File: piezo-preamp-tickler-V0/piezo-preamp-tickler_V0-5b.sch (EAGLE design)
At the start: 22 parts, among them IC1 TLC272, Q4 2N5484

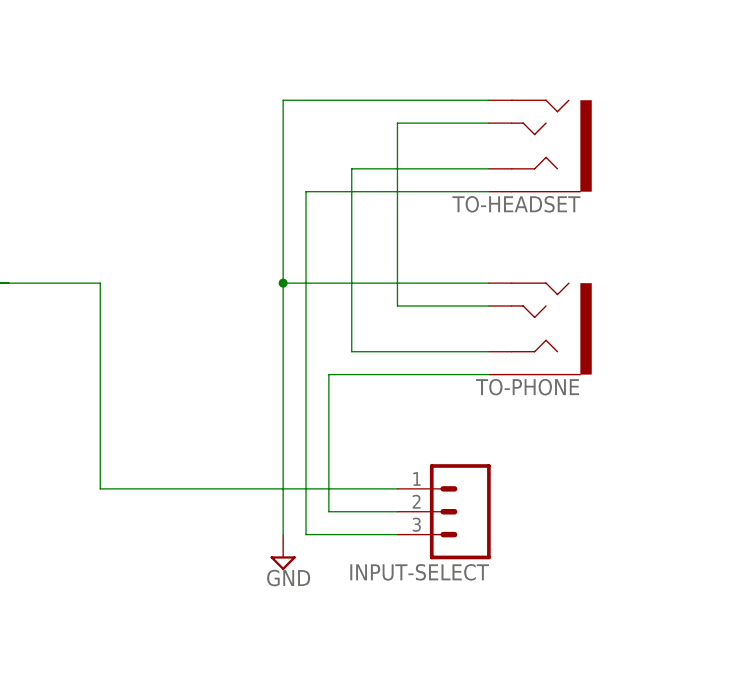
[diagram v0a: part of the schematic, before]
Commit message: changes to piezo-preamp-tickler-V0-5
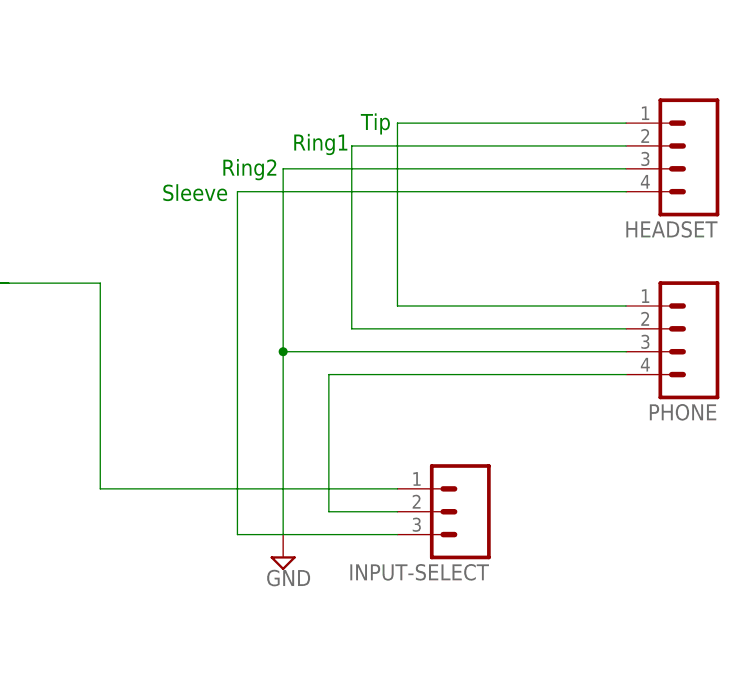
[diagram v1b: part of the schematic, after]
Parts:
- removed TO-HEADSET, TO-PHONE: AUDIO-JACK3, SparkFun-Connectors:AUDIO-JACK3
- added HEADSET, PHONE: (no value), CMU-ArtFab:M04LOCK
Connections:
- net GND: now also HEADSET.3, PHONE.3; no longer TO-HEADSET.RING2, TO-PHONE.RING2
- net N$12: now also HEADSET.4; no longer TO-HEADSET.EARTH
- net N$13: now also HEADSET.1, PHONE.1; no longer TO-HEADSET.TIP, TO-PHONE.TIP
- net N$15: now also HEADSET.2, PHONE.2; no longer TO-HEADSET.RING1, TO-PHONE.RING1
- net TO-PHONE: now also PHONE.4; no longer TO-PHONE.EARTH
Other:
- note added: "Ring1"
- note added: "Ring2"
- note added: "Sleeve"
- note added: "Tip"
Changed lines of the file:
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@@
 <part name="SUPPLY1" library="supply2" deviceset="GND" device=""/>
 <part name="SUPPLY2" library="supply2" deviceset="GND" device=""/>
-<part name="TO-PHONE" library="SparkFun-Connectors" deviceset="AUDIO-JACK3" device=""/>
 <part name="INPUT-SELECT" library="SparkFun-Connectors" deviceset="M03" device="LOCK"/>
-<part name="TO-HEADSET" library="SparkFun-Connectors" deviceset="AUDIO-JACK3" device=""/>
+<part name="HEADSET" library="CMU-ArtFab" deviceset="M04" device="LOCK"/>
+<part name="PHONE" library="CMU-ArtFab" deviceset="M04" device="LOCK"/>
 </parts>
 <sheets>
 <sheet>
 <plain>
+<text x="211.836" y="60.198" size="1.778" layer="91">Tip</text>
+<text x="189.738" y="52.324" size="1.778" layer="91">Sleeve</text>
+<text x="196.342" y="55.118" size="1.778" layer="91">Ring2</text>
+<text x="204.216" y="57.912" size="1.778" layer="91">Ring1</text>
 </plain>
 <instances>
@@
 <instance part="SUPPLY1" gate="GND" x="121.92" y="2.54"/>
 <instance part="SUPPLY2" gate="GND" x="203.2" y="12.7"/>
-<instance part="TO-PHONE" gate="G$1" x="231.14" y="38.1" smashed="yes" rot="R180">
-<attribute name="NAME" x="236.22" y="32.512" size="1.778" layer="95" rot="R180"/>
-</instance>
 <instance part="INPUT-SELECT" gate="G$1" x="223.52" y="17.78" rot="R180"/>
-<instance part="TO-HEADSET" gate="G$1" x="231.14" y="58.42" smashed="yes" rot="R180">
-<attribute name="NAME" x="236.22" y="52.832" size="1.778" layer="95" rot="R180"/>
-</instance>
+<instance part="HEADSET" gate="G$1" x="246.38" y="58.42" rot="R180"/>
+<instance part="PHONE" gate="G$1" x="246.38" y="38.1" rot="R180"/>
 </instances>
 <busses>
@@
 <segment>
 <pinref part="SUPPLY2" gate="GND" pin="GND"/>
-<wire x1="203.2" y1="43.18" x2="203.2" y2="15.24" width="0.1524" layer="91"/>
-<pinref part="TO-PHONE" gate="G$1" pin="RING2"/>
-<wire x1="226.06" y1="43.18" x2="203.2" y2="43.18" width="0.1524" layer="91"/>
-<wire x1="203.2" y1="43.18" x2="203.2" y2="63.5" width="0.1524" layer="91"/>
-<junction x="203.2" y="43.18"/>
-<pinref part="TO-HEADSET" gate="G$1" pin="RING2"/>
-<wire x1="203.2" y1="63.5" x2="226.06" y2="63.5" width="0.1524" layer="91"/>
+<wire x1="203.2" y1="35.56" x2="203.2" y2="15.24" width="0.1524" layer="91"/>
+<wire x1="241.3" y1="35.56" x2="203.2" y2="35.56" width="0.1524" layer="91"/>
+<wire x1="203.2" y1="35.56" x2="203.2" y2="55.88" width="0.1524" layer="91"/>
+<junction x="203.2" y="35.56"/>
+<wire x1="203.2" y1="55.88" x2="241.3" y2="55.88" width="0.1524" layer="91"/>
+<pinref part="HEADSET" gate="G$1" pin="3"/>
+<pinref part="PHONE" gate="G$1" pin="3"/>
 </segment>
 </net>
@@
 <net name="TO-PHONE" class="0">
 <segment>
-<pinref part="TO-PHONE" gate="G$1" pin="EARTH"/>
-<wire x1="226.06" y1="33.02" x2="208.28" y2="33.02" width="0.1524" layer="91"/>
+<wire x1="241.3" y1="33.02" x2="208.28" y2="33.02" width="0.1524" layer="91"/>
 <wire x1="208.28" y1="33.02" x2="208.28" y2="17.78" width="0.1524" layer="91"/>
 <pinref part="INPUT-SELECT" gate="G$1" pin="2"/>
 <wire x1="208.28" y1="17.78" x2="215.9" y2="17.78" width="0.1524" layer="91"/>
+<pinref part="PHONE" gate="G$1" pin="4"/>
 </segment>
 </net>
 <net name="N$12" class="0">
 <segment>
-<pinref part="TO-HEADSET" gate="G$1" pin="EARTH"/>
-<wire x1="226.06" y1="53.34" x2="205.74" y2="53.34" width="0.1524" layer="91"/>
-<wire x1="205.74" y1="53.34" x2="205.74" y2="15.24" width="0.1524" layer="91"/>
+<wire x1="241.3" y1="53.34" x2="198.12" y2="53.34" width="0.1524" layer="91"/>
+<wire x1="198.12" y1="53.34" x2="198.12" y2="15.24" width="0.1524" layer="91"/>
 <pinref part="INPUT-SELECT" gate="G$1" pin="3"/>
-<wire x1="205.74" y1="15.24" x2="215.9" y2="15.24" width="0.1524" layer="91"/>
+<wire x1="198.12" y1="15.24" x2="215.9" y2="15.24" width="0.1524" layer="91"/>
+<pinref part="HEADSET" gate="G$1" pin="4"/>
 </segment>
 </net>
 <net name="N$13" class="0">
 <segment>
-<pinref part="TO-PHONE" gate="G$1" pin="TIP"/>
-<wire x1="226.06" y1="40.64" x2="215.9" y2="40.64" width="0.1524" layer="91"/>
 <wire x1="215.9" y1="40.64" x2="215.9" y2="60.96" width="0.1524" layer="91"/>
-<pinref part="TO-HEADSET" gate="G$1" pin="TIP"/>
-<wire x1="215.9" y1="60.96" x2="226.06" y2="60.96" width="0.1524" layer="91"/>
+<pinref part="HEADSET" gate="G$1" pin="1"/>
+<wire x1="215.9" y1="60.96" x2="241.3" y2="60.96" width="0.1524" layer="91"/>
+<pinref part="PHONE" gate="G$1" pin="1"/>
+<wire x1="215.9" y1="40.64" x2="241.3" y2="40.64" width="0.1524" layer="91"/>
 </segment>
 </net>
 <net name="N$15" class="0">
 <segment>
-<pinref part="TO-PHONE" gate="G$1" pin="RING1"/>
-<wire x1="226.06" y1="35.56" x2="210.82" y2="35.56" width="0.1524" layer="91"/>
-<wire x1="210.82" y1="35.56" x2="210.82" y2="55.88" width="0.1524" layer="91"/>
-<pinref part="TO-HEADSET" gate="G$1" pin="RING1"/>
-<wire x1="210.82" y1="55.88" x2="226.06" y2="55.88" width="0.1524" layer="91"/>
-</segment>
-</net>
+<wire x1="241.3" y1="38.1" x2="210.82" y2="38.1" width="0.1524" layer="91"/>
+<wire x1="210.82" y1="38.1" x2="210.82" y2="58.42" width="0.1524" layer="91"/>
+<wire x1="210.82" y1="58.42" x2="241.3" y2="58.42" width="0.1524" layer="91"/>
+<pinref part="HEADSET" gate="G$1" pin="2"/>
+<pinref part="PHONE" gate="G$1" pin="2"/>
+</segment>
+</net>
